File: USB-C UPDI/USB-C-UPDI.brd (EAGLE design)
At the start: 27.4 x 18.3 mm, 9 parts, among them IC1 FT232RL, J2 61300511121

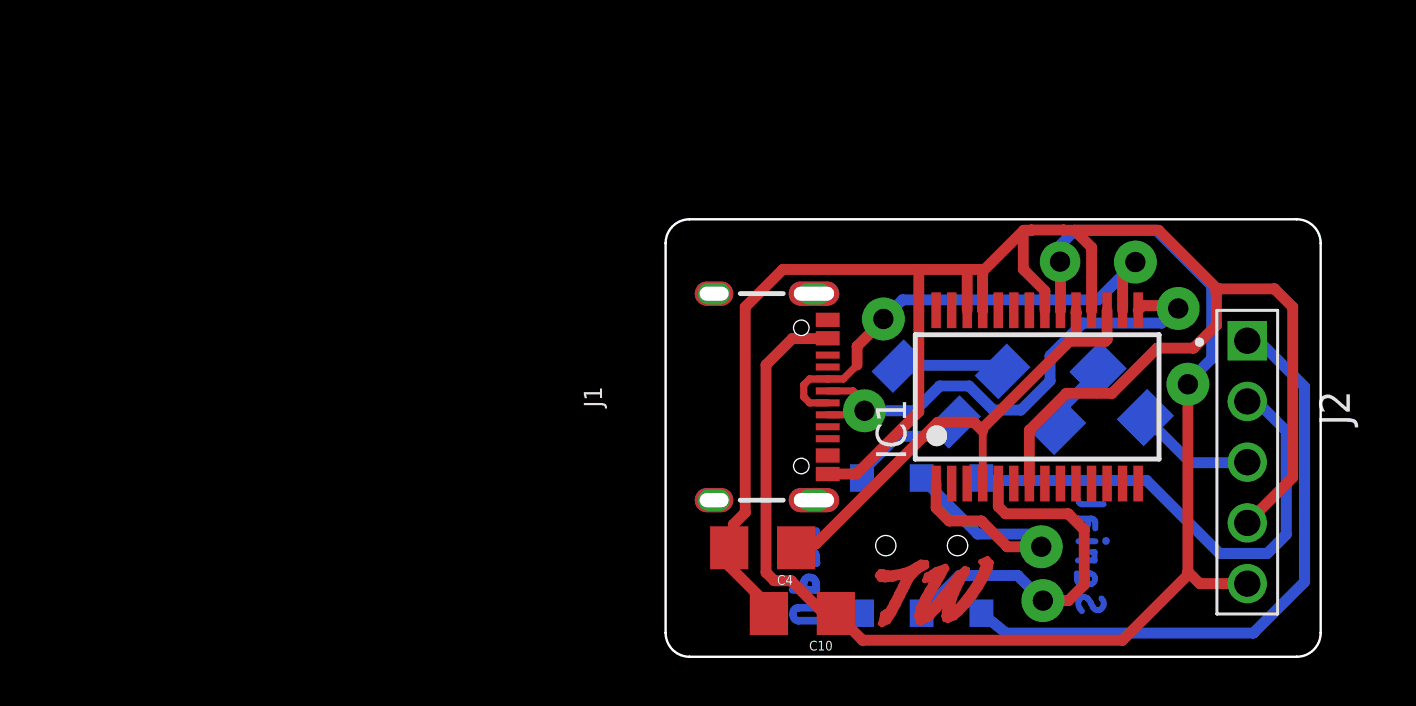
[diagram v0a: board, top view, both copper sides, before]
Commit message: updates
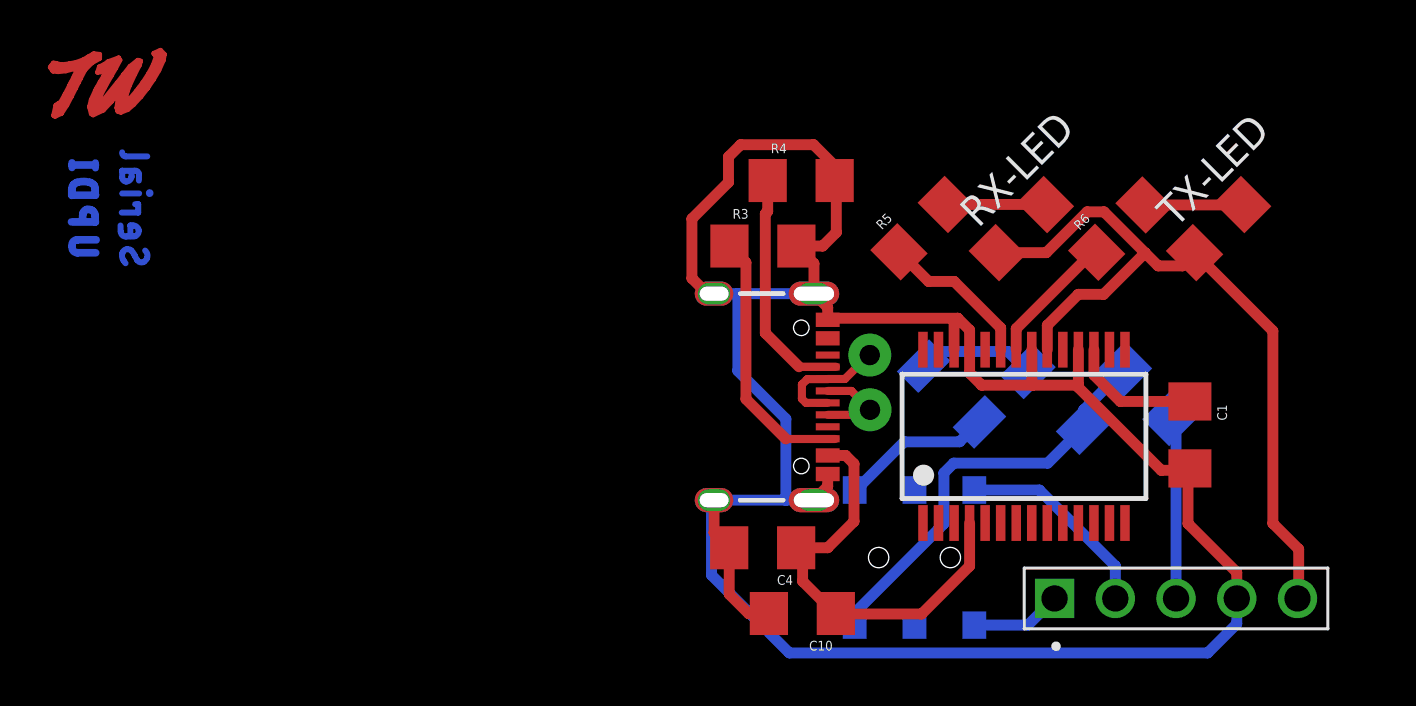
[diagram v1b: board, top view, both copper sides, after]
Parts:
- added C1: 100nf, 01_SparkFun:1206
- added R3, R4: 5.1k, 01_SparkFun:1206
- added R5, R6: 330, 01_SparkFun:1206
- added RX-LED, TX-LED: LED, eagle_fab:LED1206
- C10: value 1uf -> 4.7uf
- moved J2 6.43 mm to (21.2, 6.04), turned to 0 degrees
- moved IC1 1.74 mm to (14.9, 12.8)
- moved D1 1.06 mm to (16.2, 14.4)
- moved R1 1.06 mm to (11.9, 14.6)
- moved R2 1.06 mm to (20.0, 14.6)
- moved S1 0.58 mm to (10.3, 7.75)
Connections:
- new net N$1: C1.1, IC1.17
- new net N$42: J1.B5, R3.1
- new net N$43: IC1.22, R6.1
- new net N$44: IC1.23, R5.1
- new net N$45: R5.2, RX-LED.2
- new net N$46: R6.2, TX-LED.2
- net GND: now also C1.2, J1.SHLD1, J1.SHLD2, J1.SHLD3, J1.SHLD4, R3.2, R4.2
- net N$9: now also J1.A5, R4.1; no longer C4.1, IC1.17, IC1.19, IC1.4
- net VCC: now also C4.1, IC1.4, RX-LED.1, TX-LED.1
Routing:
- net RX: track 26.1 -> 3.82 mm
- net GND: track 84.3 -> 103.4 mm
- net N$13: track 16.3 -> 0.00 mm, vias 1 -> 0
- net N$7: track 15.4 -> 0.00 mm, vias 1 -> 0
- net N$3: track 3.35 -> 17.6 mm
- net N$10: track 12.5 -> 0.00 mm, vias 1 -> 0
- net TX: track 20.8 -> 8.58 mm
- net N$9: track 21.7 -> 9.96 mm
- net N$6: track 11.5 -> 0.00 mm
- net N$42: track 0.00 -> 11.1 mm
- net N$44: track 0.00 -> 6.48 mm
- net VCC: track 57.3 -> 51.0 mm, vias 2 -> 0
- net N$43: track 0.00 -> 5.57 mm
- net N$1: track 0.00 -> 5.53 mm
- net N$45: track 0.00 -> 4.15 mm
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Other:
- board size 27.4 x 18.3 mm -> 5 x 8.6 mm
